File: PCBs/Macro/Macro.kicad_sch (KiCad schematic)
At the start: 7 parts, among them J1 Male_Pogo_Connector_01x05, J2 Male_Pogo_Connector_01x05, J3 Male_Pogo_Connector_01x05, J4 Male_Pogo_Connector_01x05, SW1 RotaryEncoder_Switch, SW2 RotaryEncoder_Switch, U1 XIAO-RP2040-DIP

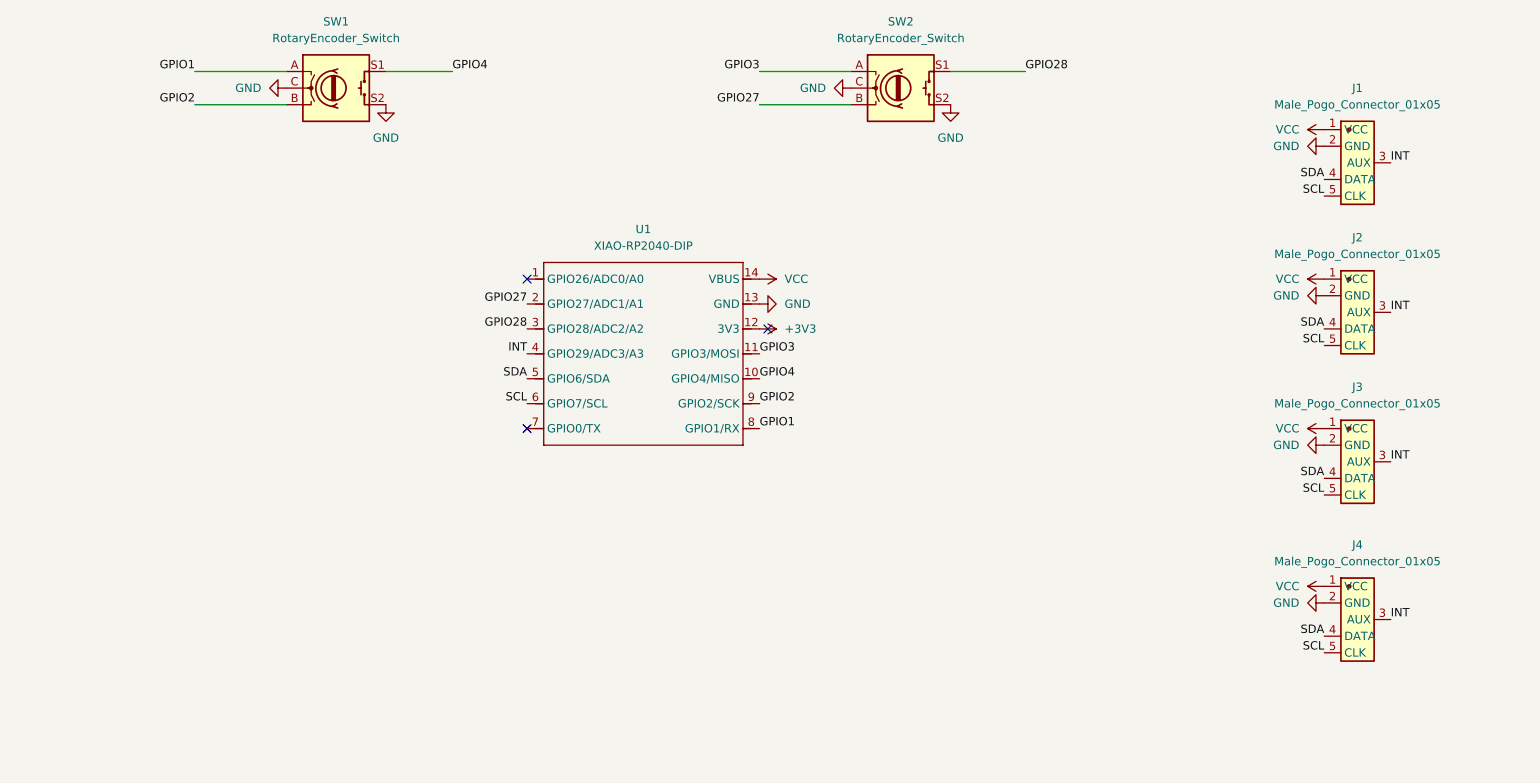
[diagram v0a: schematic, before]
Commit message: Finished Designing
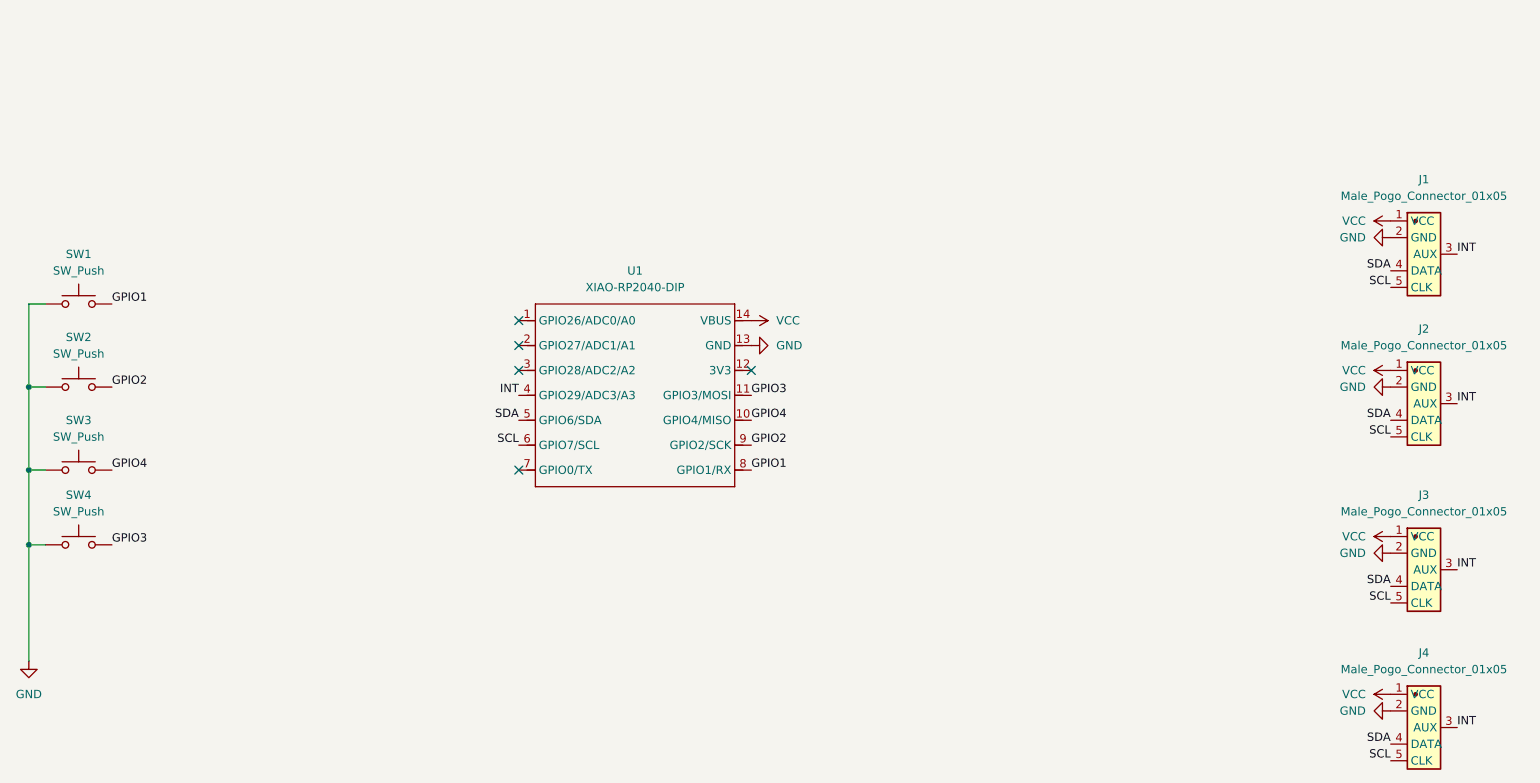
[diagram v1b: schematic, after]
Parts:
- removed SW1, SW2: RotaryEncoder_Switch, Rotary_Encoder:RotaryEncoder_Alps_EC11E-Switch_Vertical_H20mm, symbol Device:RotaryEncoder_Switch
- added SW1, SW2, SW3, SW4: SW_Push, Button_Switch_Keyboard:SW_Cherry_MX_1.00u_PCB, symbol Switch:SW_Push
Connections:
- net GND: now also SW1.1, SW2.1, SW3.1, SW4.1
- net GPIO1: now also SW1.2
- net GPIO2: now also SW2.2
- net GPIO3: now also SW4.2
- net GPIO4: now also SW3.2
- net +3V3: no longer names the net of U1.12 (3V3)
- net GPIO27: no longer names the net of U1.2 (GPIO27/ADC1/A1)
- net GPIO28: no longer names the net of U1.3 (GPIO28/ADC2/A2)
- no-connect marks 3 -> 5
